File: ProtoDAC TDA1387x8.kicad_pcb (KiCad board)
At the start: 2 copper layers, 65 x 56.5 mm, 15 parts, among them IC1 TDA1541A, J1 936, J2 936

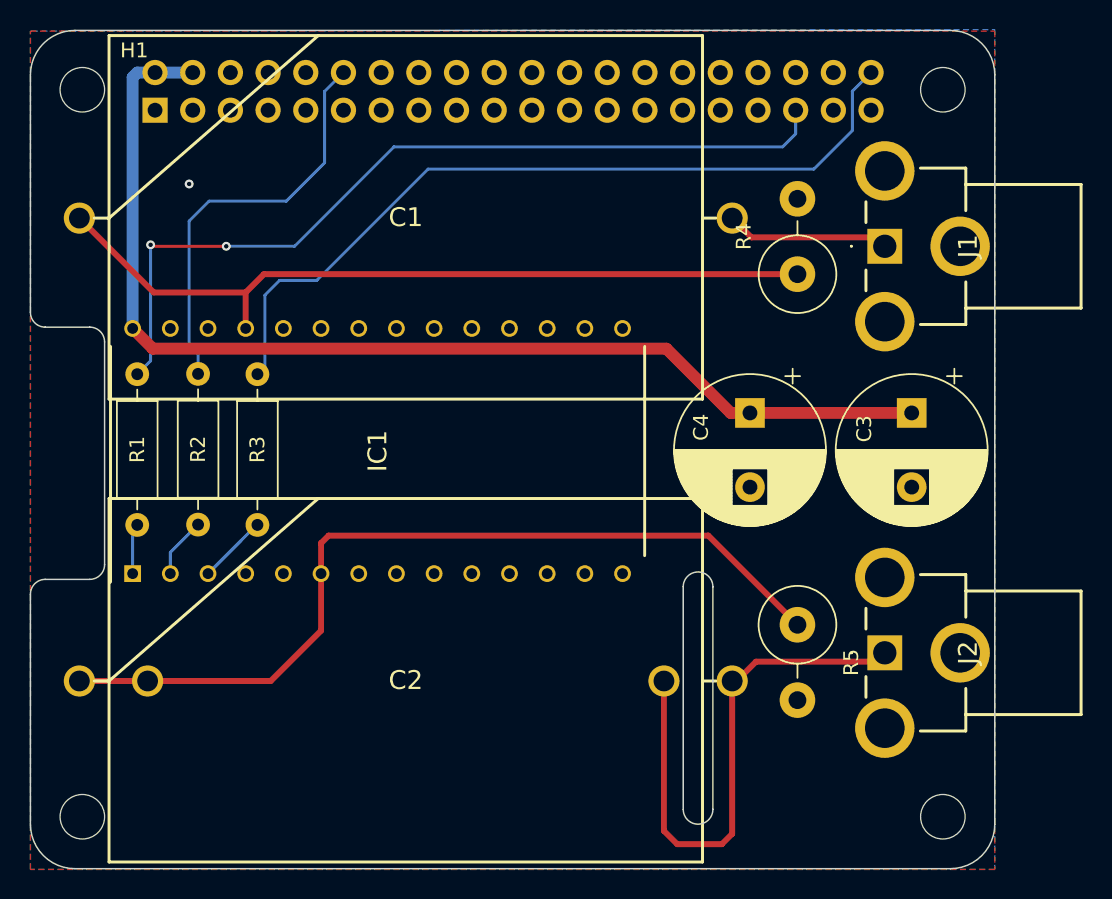
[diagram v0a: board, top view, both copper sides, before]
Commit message: Updated board to match new layout
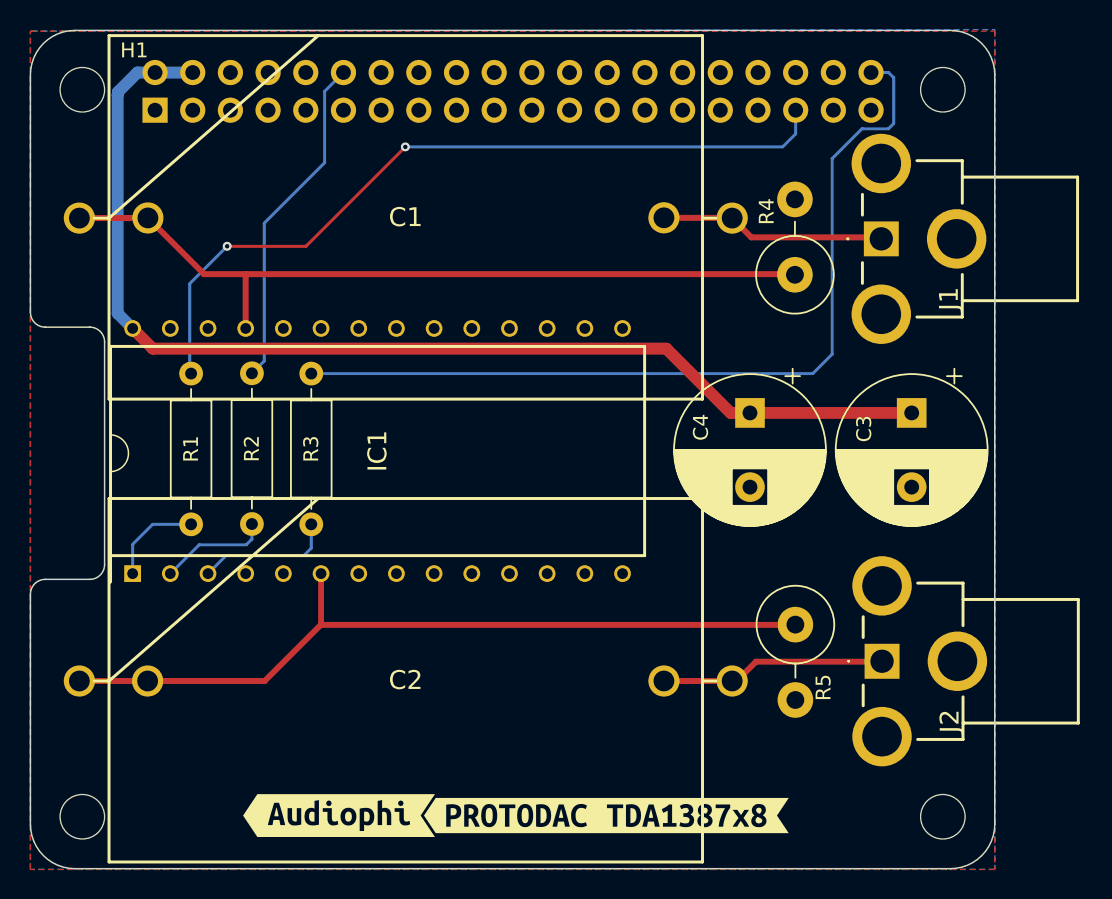
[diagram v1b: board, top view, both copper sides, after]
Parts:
- added ?: , , F.Cu at (162.2, 88.3)
- added ?: , , F.Cu at (127.4, 88.3)
- added kibuzzard-674DA88C: G***, kibuzzard-674DA88C, F.Cu at (140.3, 128.6)
- added kibuzzard-674DA90A: G***, kibuzzard-674DA90A, F.Cu at (158.3, 128.6)
- moved R1 3.63 mm to (130.3, 108.9)
- moved R2 3.63 mm to (134.4, 108.9)
- moved R3 3.63 mm to (138.4, 108.9)
- moved J2 0.60 mm to (176.9, 118.2)
- moved J1 0.55 mm to (176.8, 89.7)
- moved R4 0.17 mm to (171.0, 92.1)
- moved R5 0.14 mm to (171.1, 115.7)
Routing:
- net Net-(C2--): track 37.6 -> 17.6 mm
- net AOR: track 58.7 -> 53.5 mm
- net Net-(H1-BCM18_PCM_C): track 27.8 -> 22.8 mm
- net Net-(C1--): track 11.1 -> 15.8 mm
- net AOL: track 53.4 -> 58.1 mm
- net Net-(H1-BCM19_MISO_PCM_FS): track 57.3 -> 52.7 mm
- net Net-(H1-BCM21_SCLK_PCM_DO): track 54.2 -> 58.7 mm
- net BCK: track 4.08 -> 7.48 mm
- net LE/WS: track 3.41 -> 6.47 mm
- net DATA: track 7.84 -> 9.28 mm
- net +5V: track 76.0 -> 76.8 mm
- net GND: vias 1 -> 0
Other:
- outline, holes or cut-outs redrawn
